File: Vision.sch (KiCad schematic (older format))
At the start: 141 parts, among them J1 Conn_ARM_JTAG_SWD_10, Q1 DTC123J, SW1 SW_Push, U1 MCP1700-3002E_SOT23, U2 STM32F072CBUx, U3 TPD4E05U06DQAR

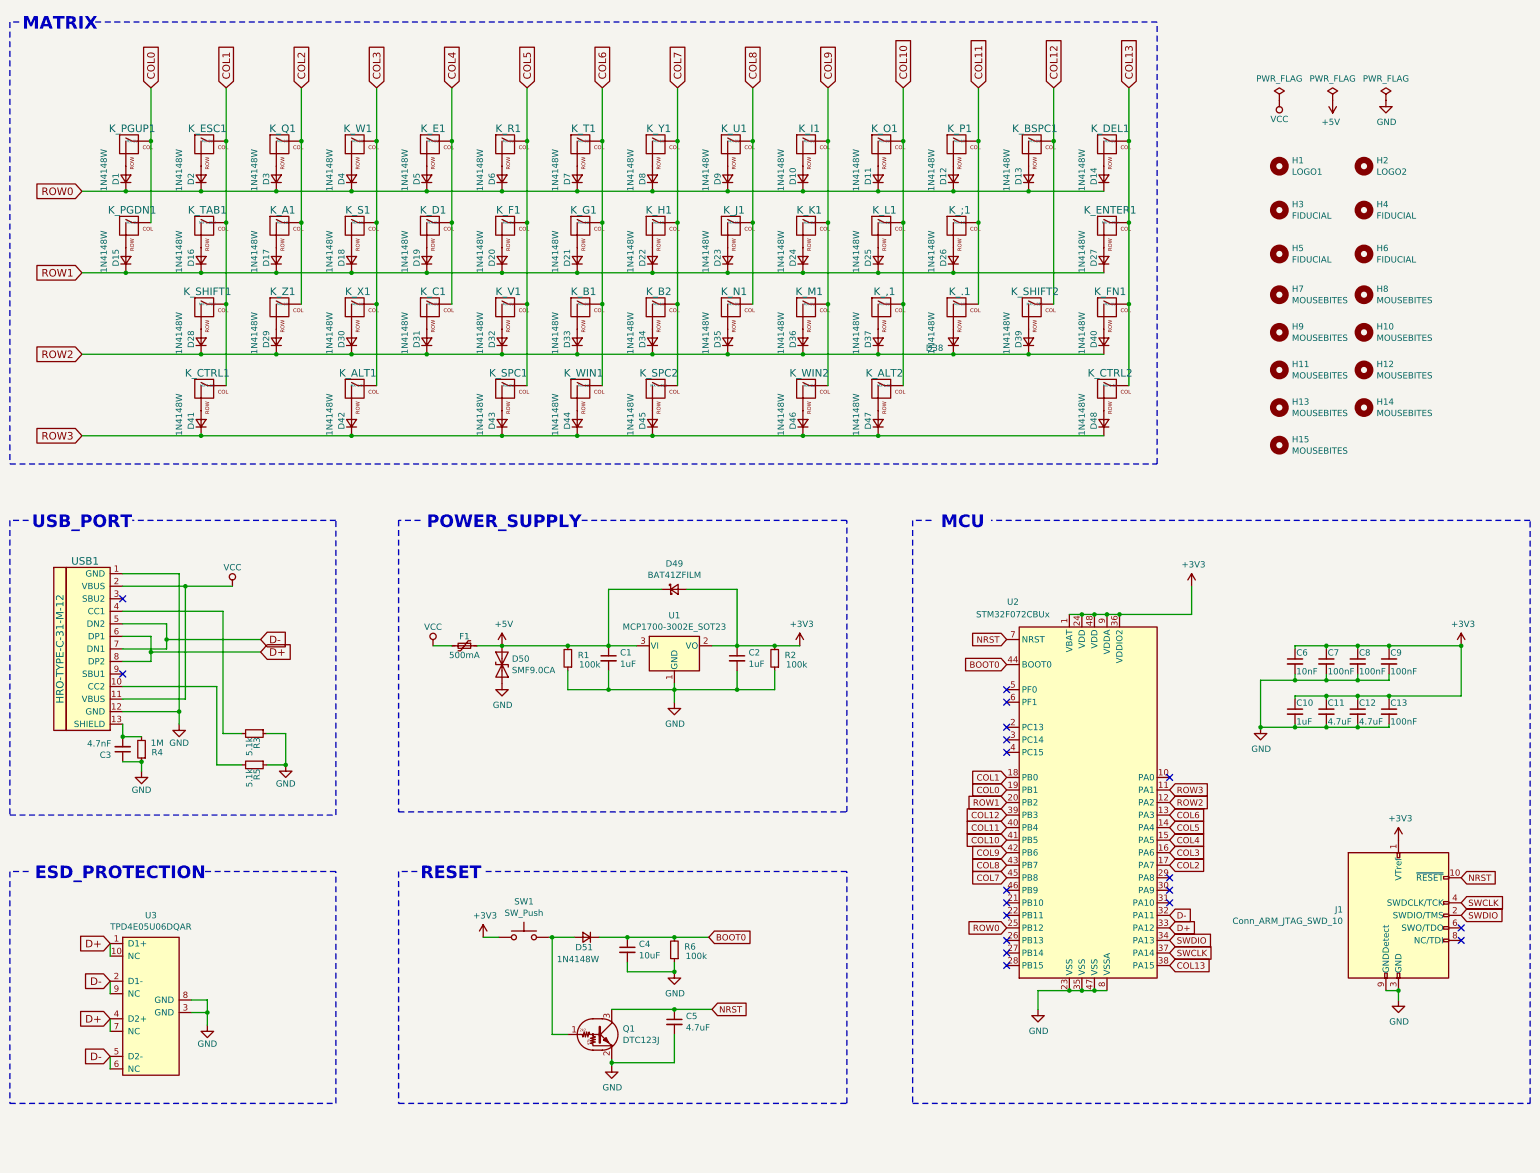
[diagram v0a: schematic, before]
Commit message: Update schematics
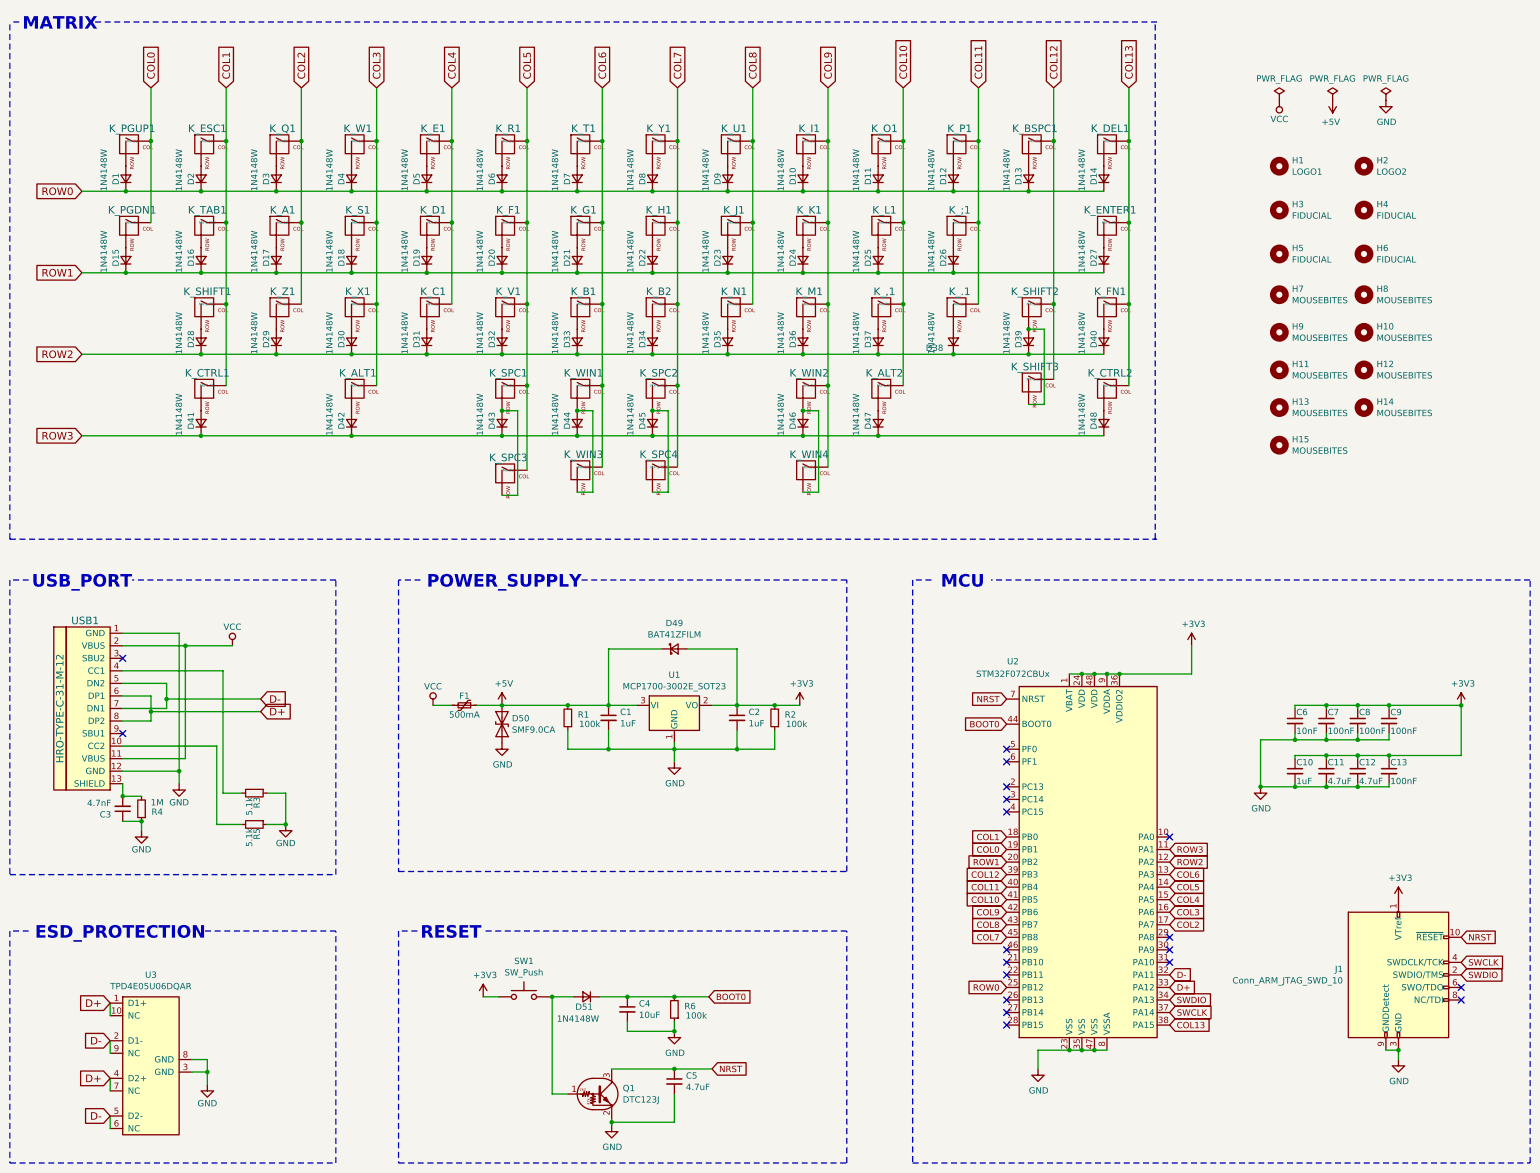
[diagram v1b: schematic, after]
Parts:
- added K_SHIFT3: MX-1.25U, MX_Only:MXOnly-2.25U-NoLED, symbol MX_Alps_Hybrid:MX-NoLED
- added K_SPC3: MX-2U, MX_Only:MXOnly-1.75U-NoLED, symbol MX_Alps_Hybrid:MX-NoLED
- added K_SPC4: MX-1.75U, MX_Only:MXOnly-1U-NoLED, symbol MX_Alps_Hybrid:MX-NoLED
- added K_WIN3: MX-1U, MX_Only:MXOnly-1.25U-NoLED, symbol MX_Alps_Hybrid:MX-NoLED
- added K_WIN4: MX-1U, MX_Only:MXOnly-1.75U-NoLED, symbol MX_Alps_Hybrid:MX-NoLED
- K_,1, K_.1, K_;1, K_A1, K_B1, K_B2, K_BSPC1, K_C1, K_D1, K_DEL1, K_E1, K_ESC1, K_F1, K_FN1, K_G1, K_H1, K_I1, K_J1, K_K1, K_L1, K_M1, K_N1, K_O1, K_P1, K_PGDN1, K_PGUP1, K_Q1, K_R1, K_S1, K_T1, K_U1, K_V1, K_W1, K_WIN1, K_WIN2, K_X1, K_Y1, K_Z1: footprint MX_Only:MXOnly-1U-Hotswap -> MX_Only:MXOnly-1U-NoLED
- K_ALT1, K_ALT2, K_CTRL1, K_CTRL2: footprint MX_Only:MXOnly-1.5U-Hotswap -> MX_Only:MXOnly-1.5U-NoLED
- K_ENTER1, K_SHIFT1: footprint MX_Only:MXOnly-1.75U-Hotswap -> MX_Only:MXOnly-1.75U-NoLED
- K_SHIFT2, K_TAB1: footprint MX_Only:MXOnly-1.25U-Hotswap -> MX_Only:MXOnly-1.25U-NoLED
- K_SPC1: footprint MX_Only:MXOnly-2U-Hotswap-ReversedStabilizers -> MX_Only:MXOnly-2U-ReversedStabilizers-NoLED
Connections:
- net COL12: now also K_SHIFT3.1 (COL)
- net COL5: now also K_SPC3.1 (COL)
- net COL6: now also K_WIN3.1 (COL)
- net COL7: now also K_SPC4.1 (COL)
- net COL9: now also K_WIN4.1 (COL)
- net at D39.2 (A), K_SHIFT2.2 (ROW): now also K_SHIFT3.2 (ROW)
- net at D45.2 (A), K_SPC2.2 (ROW): now also K_SPC4.2 (ROW)
- net at D43.2 (A), K_SPC1.2 (ROW): now also K_SPC3.2 (ROW)
- net at D44.2 (A), K_WIN1.2 (ROW): now also K_WIN3.2 (ROW)
- net at D46.2 (A), K_WIN2.2 (ROW): now also K_WIN4.2 (ROW)
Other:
- moved on the sheet: C1, C10, C11, C12, C13, C2, C3, C4, C5, C6, C7, C8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

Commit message: Update PCB
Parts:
- K_SPC2: footprint MX_Only:MXOnly-1.75U-Hotswap -> MX_Only:MXOnly-1.75U-NoLED
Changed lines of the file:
@@
 F 0 "K_SPC2" H 6025 4125 60  0000 C CNN
 F 1 "MX-1.75U" H 6025 4025 20  0000 C CNN
-F 2 "MX_Only:MXOnly-1.75U-Hotswap" H 6000 3950 60  0001 C CNN
+F 2 "MX_Only:MXOnly-1.75U-NoLED" H 6000 3950 60  0001 C CNN
 F 3 "" H 6000 3950 60  0001 C CNN
 	1    6025 3975
